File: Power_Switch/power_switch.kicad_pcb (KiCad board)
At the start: 2 copper layers, 13 x 18.5 mm, 3 parts, among them J1 Conn_01x02_Pin, J2 Conn_01x02_Socket, SW1 SW_SPDT

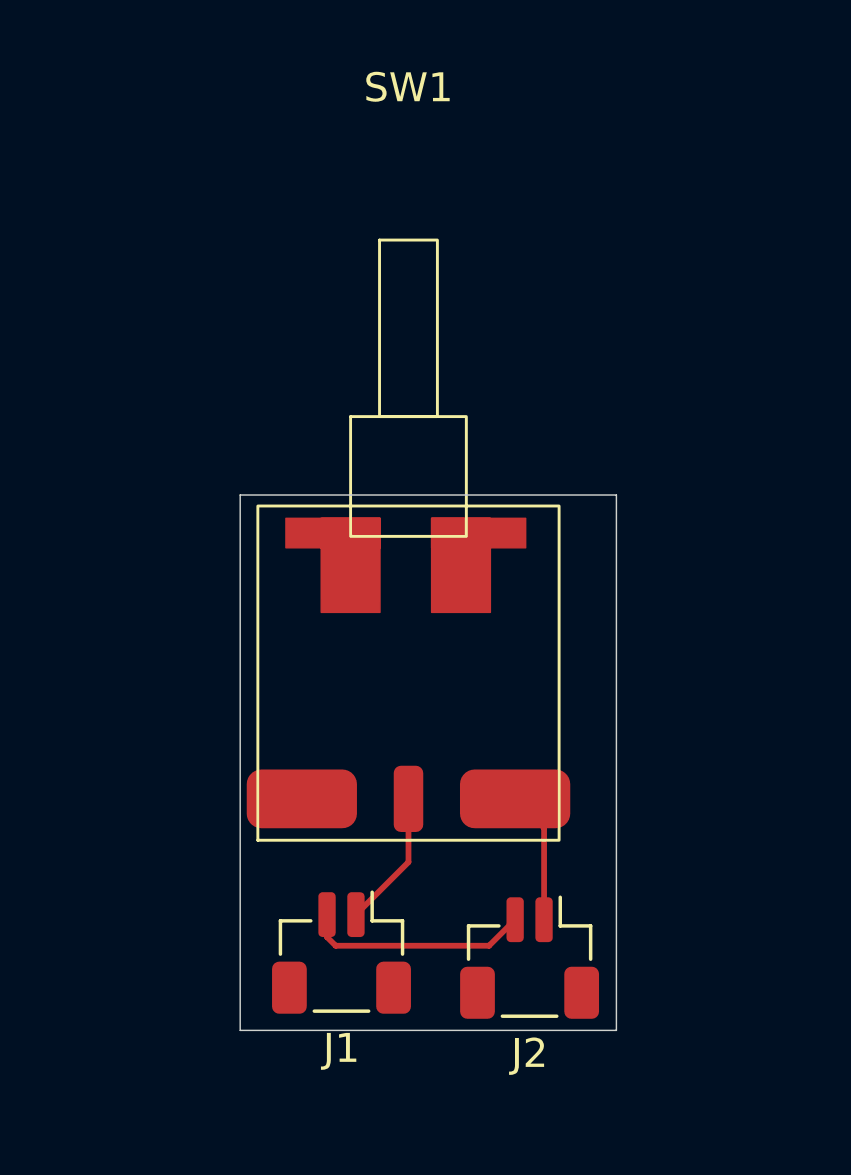
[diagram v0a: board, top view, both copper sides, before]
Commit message: small changes - probably wont use
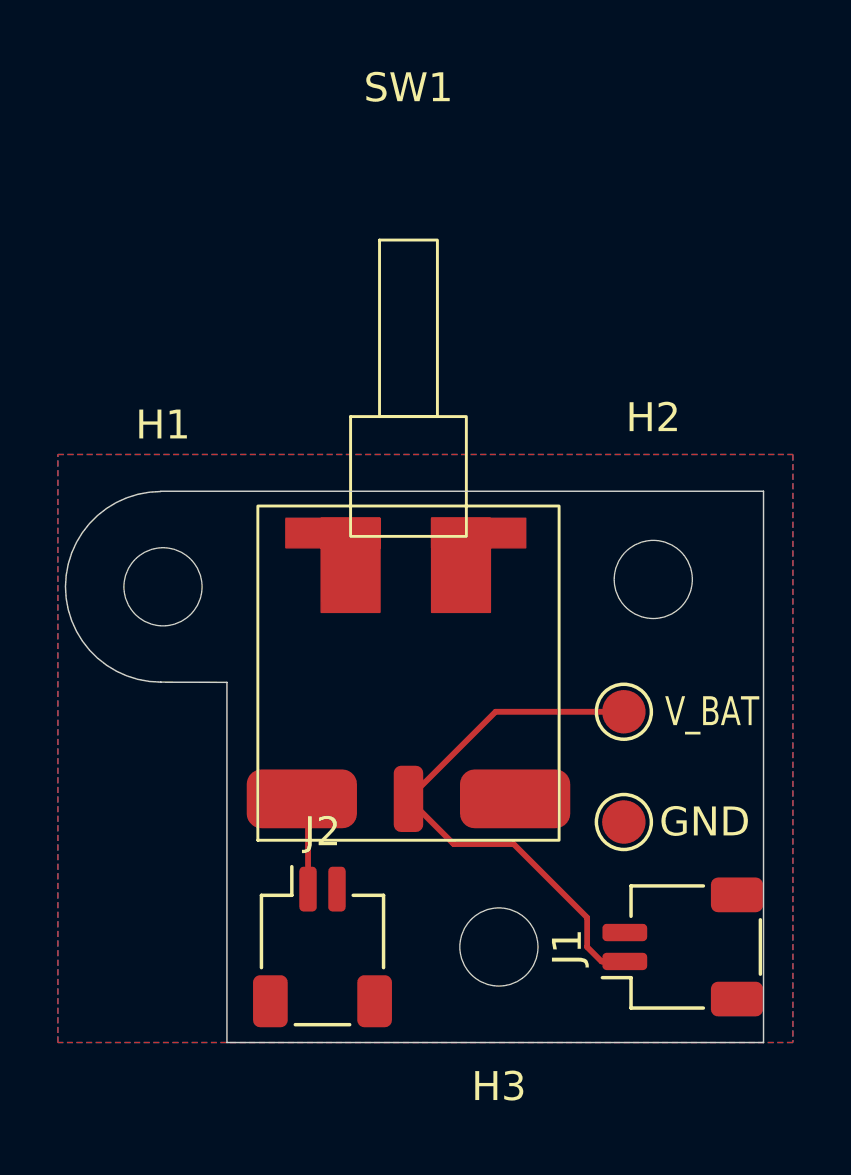
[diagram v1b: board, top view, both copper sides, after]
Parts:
- added GND: TestPoint, TestPoint:TestPoint_Pad_D1.5mm, F.Cu at (159.3, 50.8)
- added H1: MountingHole, MountingHole:MountingHole_2.7mm_M2.5, F.Cu at (143.3, 42.7)
- added H2: MountingHole, MountingHole:MountingHole_2.7mm_M2.5, F.Cu at (160.3, 42.4)
- added H3: MountingHole, MountingHole:MountingHole_2.7mm_M2.5, F.Cu at (154.9, 55.1)
- added V_BAT: TestPoint, TestPoint:TestPoint_Pad_D1.5mm, F.Cu at (159.3, 47.0)
- J1, J2: footprint Connector_JST:JST_SH_BM02B-SRSS-TB_1x02-1MP_P1.00mm_Vertical -> Connector_JST:JST_SH_SM02B-SRSS-TB_1x02-1MP_P1.00mm_Horizontal
- moved J1 11.8 mm to (161.3, 55.1), turned to 90 degrees
- moved J2 7.17 mm to (148.8, 55.1), turned to 0 degrees
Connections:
- net Net-(J1-Pin_1) renamed /V_BAT
- net Net-(J1-Pin_2) renamed GND
- J2 pad 1: Net-(J2-Pin_1) -> /V_BAT_SWITCHED
- SW1 pad 1: unconnected-(SW1-A-Pad1) -> /V_BAT_SWITCHED
- SW1 pad 3: Net-(J2-Pin_1) -> unconnected-(SW1-C-Pad3)
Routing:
- net /V_BAT: track 4.75 -> 19.1 mm
- net GND: track 7.77 -> 0.00 mm
- net Net-(J2-Pin_1): track 4.59 -> 0.00 mm
- net /V_BAT_SWITCHED: track 0.00 -> 3.21 mm
- added copper zone on B.Cu, net GND
- added copper zone on F.Cu, net GND
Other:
- board size 13 x 18.5 mm -> 24.1 x 19.1 mm
